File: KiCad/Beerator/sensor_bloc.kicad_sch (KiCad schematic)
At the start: 19 parts

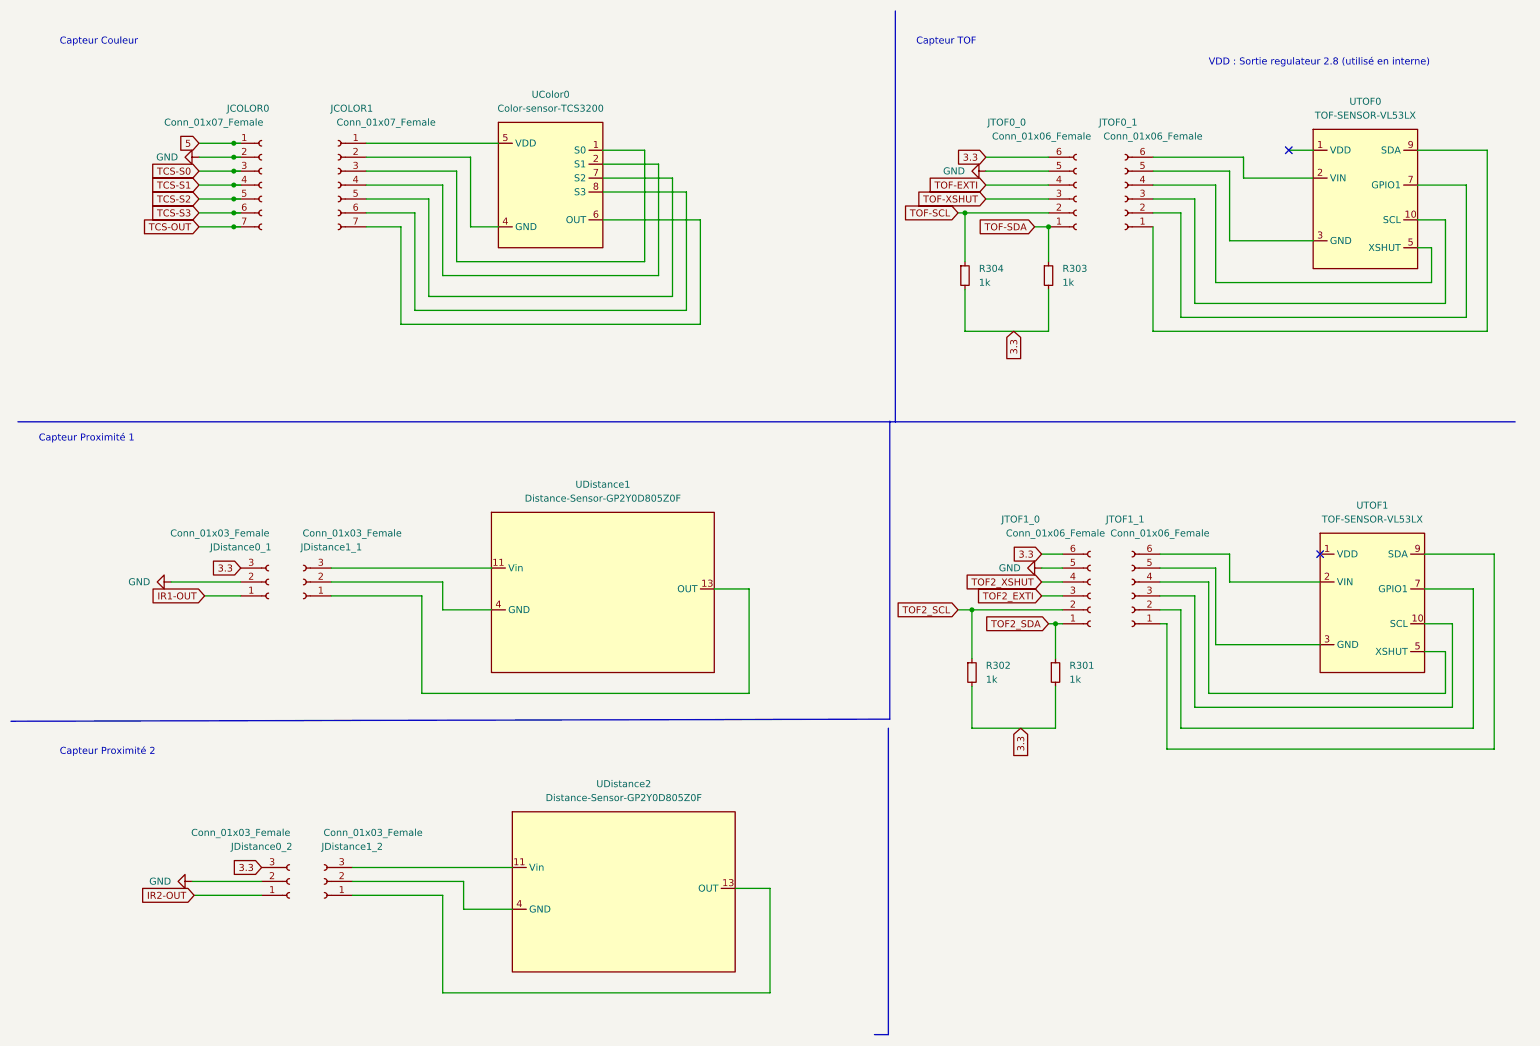
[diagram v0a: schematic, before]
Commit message: Update_Schemas
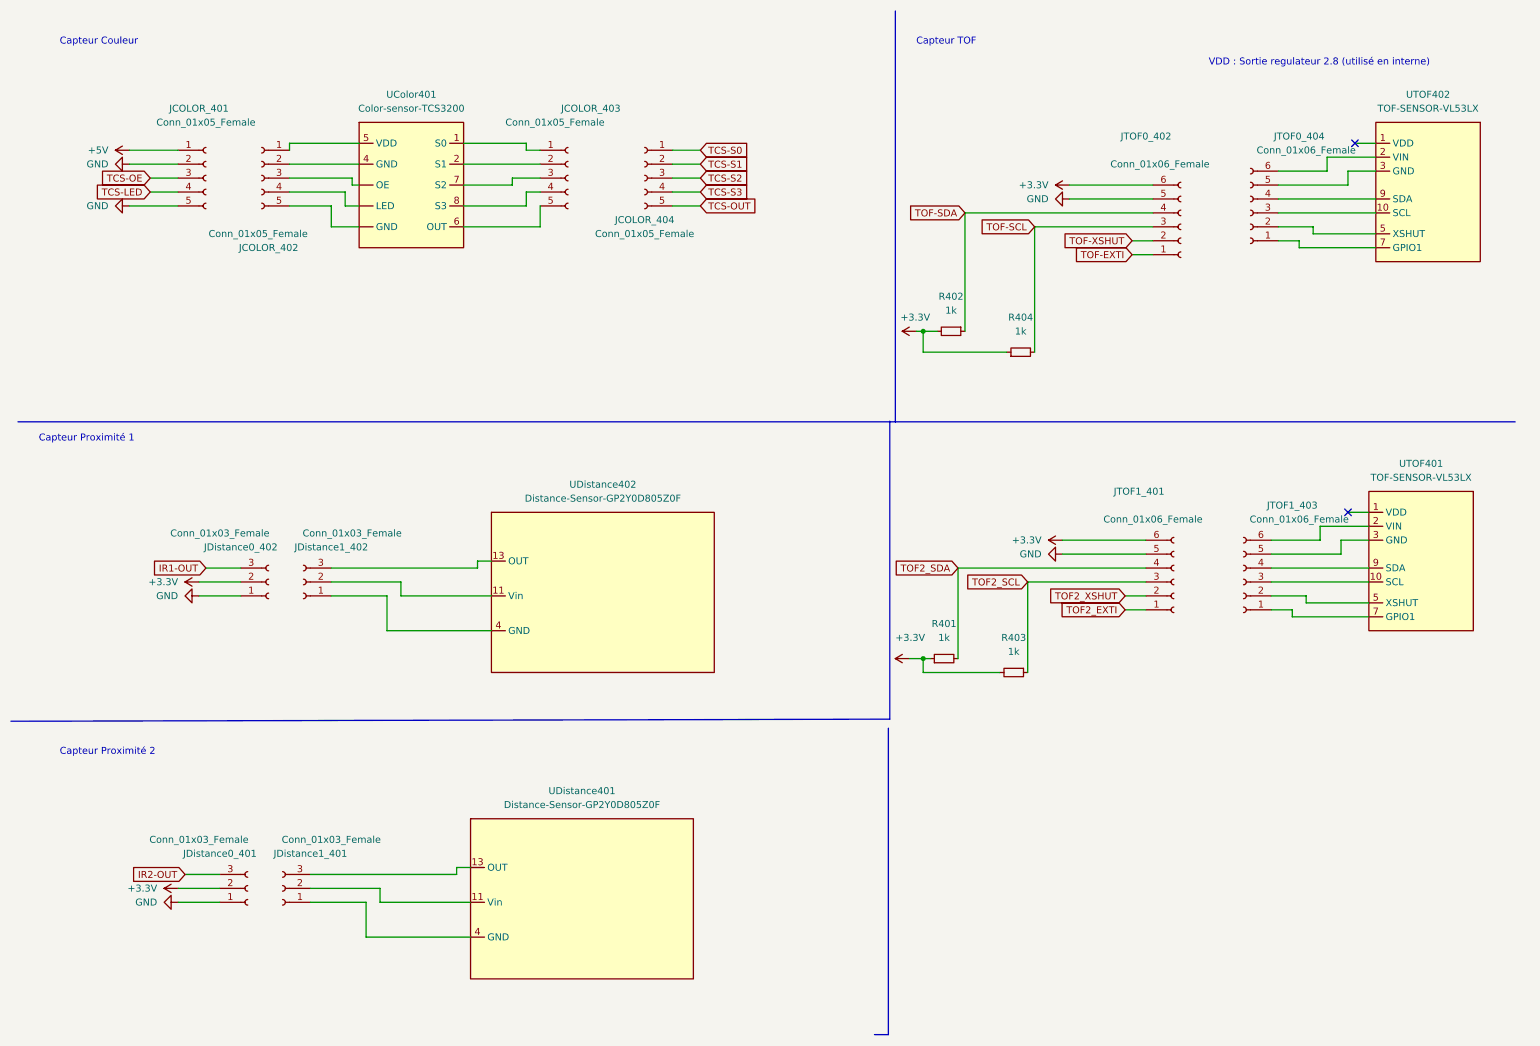
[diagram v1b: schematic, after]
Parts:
- removed JCOLOR0: Conn_01x07_Female, Connector_JST:JST_XH_B7B-XH-AM_1x07_P2.50mm_Vertical, symbol Connector:Conn_01x07_Female
- removed JCOLOR1: Conn_01x07_Female, symbol Connector:Conn_01x07_Female
- removed JDistance0_2: Conn_01x03_Female, Connector_JST:JST_XH_B3B-XH-AM_1x03_P2.50mm_Vertical, symbol Connector:Conn_01x03_Female
- removed JDistance1_2: Conn_01x03_Female, symbol Connector:Conn_01x03_Female
- removed JTOF1_0: Conn_01x06_Female, Connector_JST:JST_XH_B6B-XH-AM_1x06_P2.50mm_Vertical, symbol Connector:Conn_01x06_Female
- removed JTOF1_1: Conn_01x06_Female, symbol Connector:Conn_01x06_Female
- removed R301, R302: 1k, Resistor_SMD:R_0603_1608Metric_Pad0.98x0.95mm_HandSolder, symbol Device:R_Small
- removed UDistance2: Distance-Sensor-GP2Y0D805Z0F, symbol Sensors_Beerator:Distance-Sensor-GP2Y0D805Z0F
- removed UTOF1: TOF-SENSOR-VL53LX, symbol Sensors_Beerator:TOF-SENSOR-VL53LX
- added JCOLOR_401, JCOLOR_403: Conn_01x05_Female, Connector_JST:JST_XH_B5B-XH-AM_1x05_P2.50mm_Vertical, symbol Connector:Conn_01x05_Female
- added JCOLOR_402, JCOLOR_404: Conn_01x05_Female, symbol Connector:Conn_01x05_Female
- added JDistance0_401: Conn_01x03_Female, Connector_JST:JST_XH_B3B-XH-AM_1x03_P2.50mm_Vertical, symbol Connector:Conn_01x03_Female
- added JDistance1_401: Conn_01x03_Female, symbol Connector:Conn_01x03_Female
- added JTOF1_401: Conn_01x06_Female, Connector_JST:JST_XH_B6B-XH-AM_1x06_P2.50mm_Vertical, symbol Connector:Conn_01x06_Female
- added JTOF1_403: Conn_01x06_Female, symbol Connector:Conn_01x06_Female
- added R401, R403: 1k, Resistor_SMD:R_0603_1608Metric_Pad0.98x0.95mm_HandSolder, symbol Device:R_Small
- added UDistance401: Distance-Sensor-GP2Y0D805Z0F, symbol Sensors_Beerator:Distance-Sensor-GP2Y0D805Z0F
- added UTOF401: TOF-SENSOR-VL53LX, symbol Sensors_Beerator:TOF-SENSOR-VL53LX
- renumbered JDistance0_1 to JDistance0_402, JDistance1_1 to JDistance1_402, JTOF0_0 to JTOF0_402, JTOF0_1 to JTOF0_404, R304 to R402, R303 to R404, UColor0 to UColor401, UDistance1 to UDistance402, UTOF0 to UTOF402
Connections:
- net GND: now also JDistance0_402.1 (Pin_1), JCOLOR_401.2 (Pin_2), JCOLOR_401.5 (Pin_5), JDistance0_401.1 (Pin_1), JTOF1_401.5 (Pin_5); no longer JDistance0_402.2 (Pin_2)
- net IR1-OUT: now also JDistance0_402.3 (Pin_3); no longer JDistance0_402.1 (Pin_1)
- net IR2-OUT: now also JDistance0_401.3 (Pin_3)
- net TCS-OUT: now also JCOLOR_404.5 (Pin_5)
- net TCS-S0: now also JCOLOR_404.1 (Pin_1)
- net TCS-S1: now also JCOLOR_404.2 (Pin_2)
- net TCS-S2: now also JCOLOR_404.3 (Pin_3)
- net TCS-S3: now also JCOLOR_404.4 (Pin_4)
- net TOF-EXTI: now also JTOF0_402.1 (Pin_1); no longer JTOF0_402.4 (Pin_4)
- net TOF-SCL: now also JTOF0_402.3 (Pin_3), R404.2; no longer JTOF0_402.2 (Pin_2), R402.1
- net TOF-SDA: now also JTOF0_402.4 (Pin_4), R402.1; no longer JTOF0_402.1 (Pin_1), R404.1
- net TOF-XSHUT: now also JTOF0_402.2 (Pin_2); no longer JTOF0_402.3 (Pin_3)
- net TOF2_EXTI: now also JTOF1_401.1 (Pin_1)
- net TOF2_SCL: now also JTOF1_401.3 (Pin_3), R403.1
- net TOF2_SDA: now also JTOF1_401.4 (Pin_4), R401.2
- net TOF2_XSHUT: now also JTOF1_401.2 (Pin_2)
- net at UDistance402.11 (Vin): now also JDistance1_402.2 (Pin_2); no longer JDistance1_402.3 (Pin_3)
- net at UDistance402.13 (OUT): now also JDistance1_402.3 (Pin_3); no longer JDistance1_402.1 (Pin_1)
- net at UDistance402.4 (GND): now also JDistance1_402.1 (Pin_1); no longer JDistance1_402.2 (Pin_2)
- net at UColor401.5 (VDD): now also JCOLOR_402.1 (Pin_1)
- net at UColor401.4 (GND): now also JCOLOR_402.2 (Pin_2)
- net at UColor401.1 (S0): now also JCOLOR_403.1 (Pin_1)
- net at UColor401.2 (S1): now also JCOLOR_403.2 (Pin_2)
- net at UColor401.7 (S2): now also JCOLOR_403.3 (Pin_3)
- net at UColor401.8 (S3): now also JCOLOR_403.4 (Pin_4)
- net at UColor401.6 (OUT): now also JCOLOR_403.5 (Pin_5)
- net at JTOF0_404.1 (Pin_1): now also UTOF402.7 (GPIO1); no longer UTOF402.9 (SDA)
- net at JTOF0_404.2 (Pin_2): now also UTOF402.5 (XSHUT); no longer UTOF402.7 (GPIO1)
- net at JTOF0_404.4 (Pin_4): now also UTOF402.9 (SDA); no longer UTOF402.5 (XSHUT)
- net 3.3 renamed +3.3V
- net +3.3V: now also JDistance0_402.2 (Pin_2), R404.1, JDistance0_401.2 (Pin_2), JTOF1_401.6 (Pin_6), R401.1, R403.2; no longer JDistance0_402.3 (Pin_3), R404.2
- new net: JDistance1_401.2 (Pin_2), UDistance401.11 (Vin)
- new net: JDistance1_401.3 (Pin_3), UDistance401.13 (OUT)
- new net: JDistance1_401.1 (Pin_1), UDistance401.4 (GND)
- new net: JTOF1_403.1 (Pin_1), UTOF401.7 (GPIO1)
- new net: JTOF1_403.2 (Pin_2), UTOF401.5 (XSHUT)
- new net: JTOF1_403.3 (Pin_3), UTOF401.10 (SCL)
- new net: JTOF1_403.4 (Pin_4), UTOF401.9 (SDA)
- new net: JTOF1_403.5 (Pin_5), UTOF401.3 (GND)
- new net: JTOF1_403.6 (Pin_6), UTOF401.2 (VIN)
- new net: JCOLOR_402.3 (Pin_3), UColor401. (OE)
- new net: JCOLOR_402.4 (Pin_4), UColor401. (OE)
- new net: JCOLOR_402.5 (Pin_5), UColor401. (OE)
- new net +5V: JCOLOR_401.1 (Pin_1)
- new net TCS-LED: JCOLOR_401.4 (Pin_4)
- new net TCS-OE: JCOLOR_401.3 (Pin_3)
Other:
- moved on the sheet: JTOF0_402, JTOF0_404, R402, R404, UTOF402

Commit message: pcb_v2
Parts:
- JCOLOR_403: footprint Connector_JST:JST_XH_B5B-XH-AM_1x05_P2.50mm_Vertical -> (none)
- JCOLOR_404: footprint (none) -> Connector_JST:JST_XH_B5B-XH-AM_1x05_P2.50mm_Vertical
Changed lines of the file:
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@@
     (property "Reference" "JCOLOR_404" (id 0) (at 125.73 49.53 0))
     (property "Value" "Conn_01x05_Female" (id 1) (at 125.73 52.07 0))
-    (property "Footprint" "" (id 2) (at 125.73 41.91 0)
+    (property "Footprint" "Connector_JST:JST_XH_B5B-XH-AM_1x05_P2.50mm_Vertical" (id 2) (at 125.73 41.91 0)
       (effects (font (size 1.27 1.27)) hide)
     )
@@
       (effects (font (size 1.27 1.27)) (justify left))
     )
-    (property "Footprint" "Connector_JST:JST_XH_B5B-XH-AM_1x05_P2.50mm_Vertical" (id 2) (at 111.76 41.91 0)
-      (effects (font (size 1.27 1.27)) hide)
-    )
+    (property "Footprint" "" (id 2) (at 111.76 41.91 0)
+      (effects (font (size 1.27 1.27)) hide)
+    )
